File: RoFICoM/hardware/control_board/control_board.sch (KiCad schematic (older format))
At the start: 26 parts, among them J1 Skirt Cable, J2 M+, J3 M-, J4 SWD, J5 DBG_UART, J6 SYS_CON, J7 SLIDER, U1 STM32G071GBU6, U2 DRV8837C, U3 BU52272NUZ, U4 MIC5365, U5 BU52272NUZ

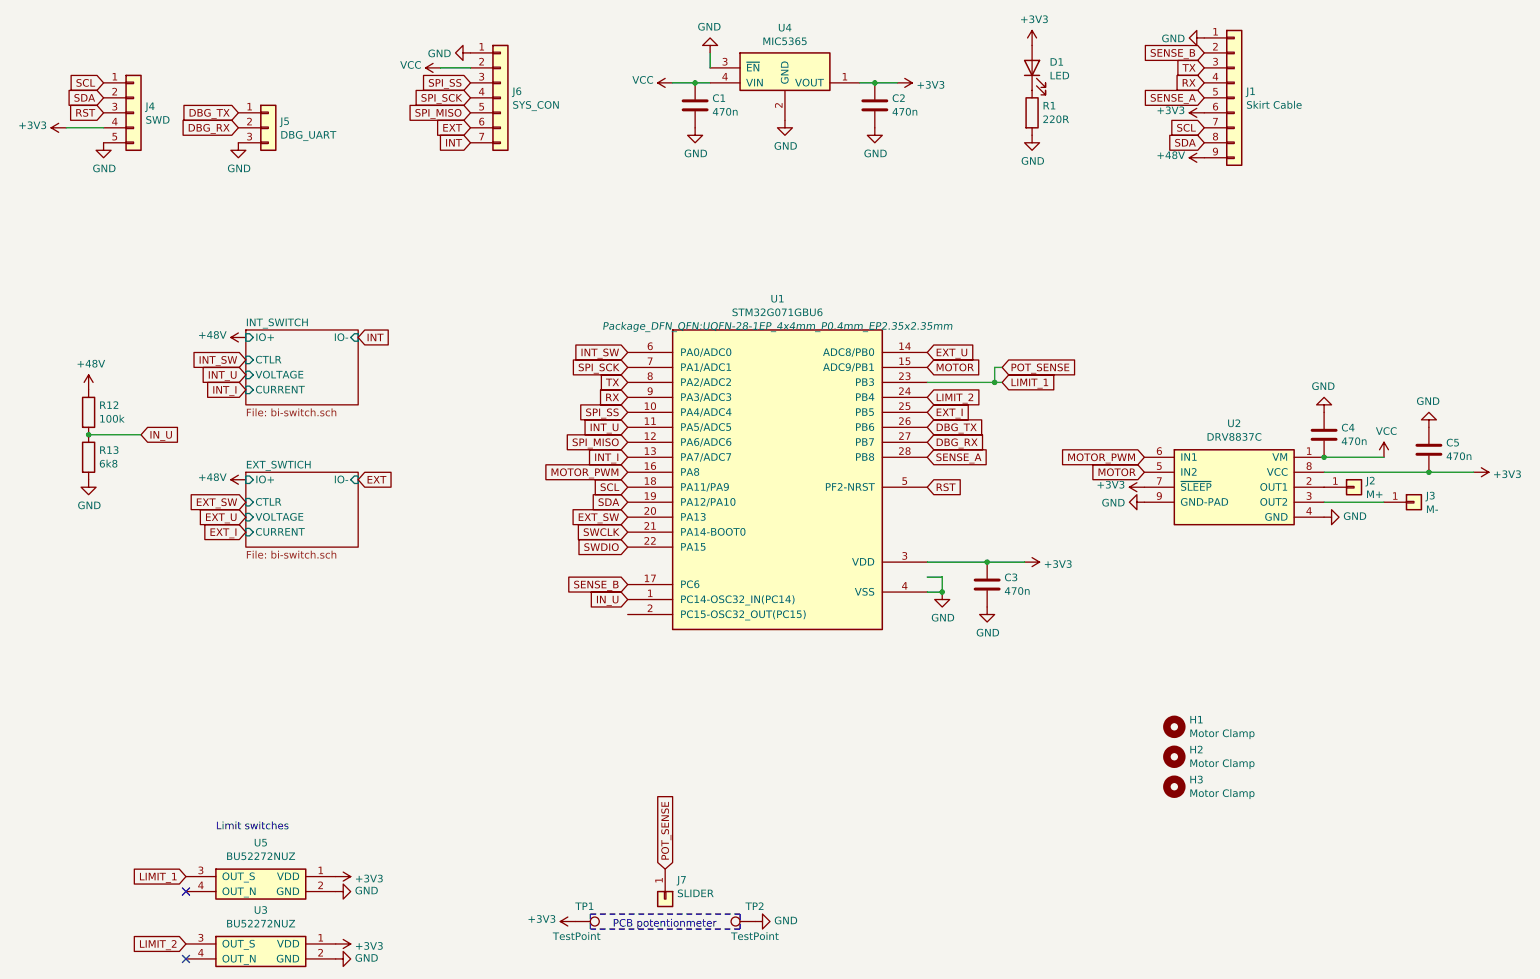
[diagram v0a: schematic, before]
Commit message: RoFICoM: Route ContorlBoard v0.2
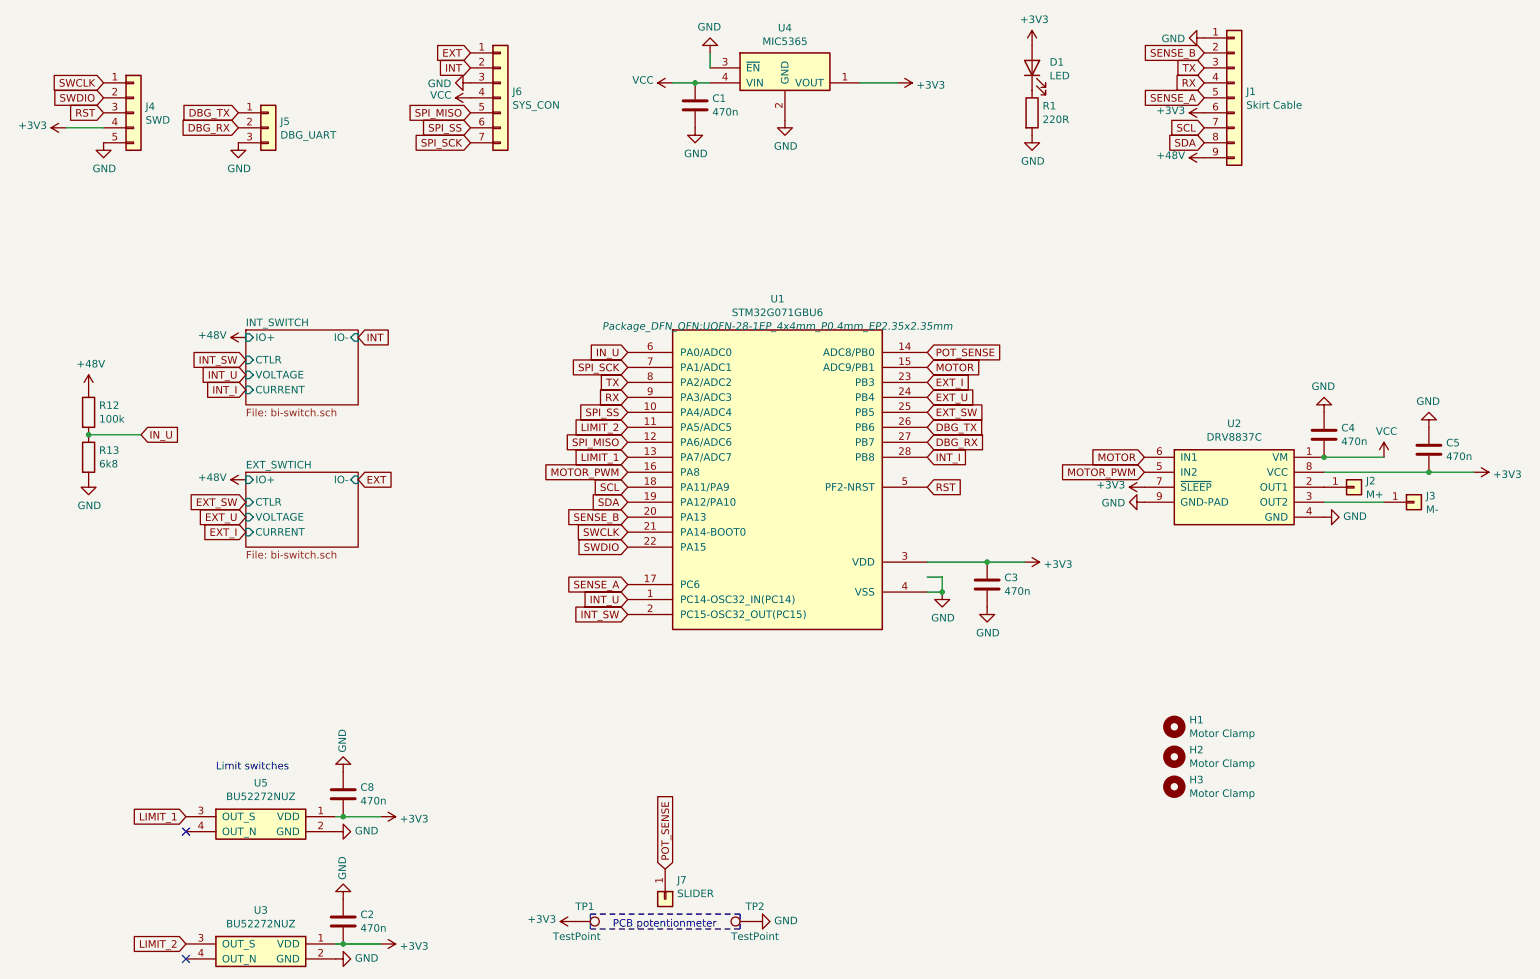
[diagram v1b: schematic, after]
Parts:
- added C8: 470n, Capacitor_SMD:C_0402_1005Metric, symbol Device:C
- J4: footprint Connector_PinHeader_1.27mm:PinHeader_1x05_P1.27mm_Vertical -> Connector_PinHeader_2.54mm:PinHeader_1x05_P2.54mm_Vertical
- J5: footprint Connector_PinHeader_1.27mm:PinHeader_1x03_P1.27mm_Vertical -> Connector_PinSocket_2.54mm:PinSocket_1x03_P2.54mm_Vertical
- J6: footprint Connector_PinHeader_1.27mm:PinHeader_1x07_P1.27mm_Vertical -> rofi:pogo_row_4_3
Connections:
- wire segments 21 -> 19
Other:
- moved on the sheet: C2, U5
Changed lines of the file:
@@
 L Device:C C2
 U 1 1 5C86BCA3
-P 6350 1550
-F 0 "C2" H 6465 1596 50  0000 L CNN
-F 1 "470n" H 6465 1505 50  0000 L CNN
-F 2 "Capacitor_SMD:C_0402_1005Metric" H 6388 1400 50  0001 C CNN
-F 3 "~" H 6350 1550 50  0001 C CNN
-	1    6350 1550
-	1    0    0    -1
-$EndComp
-Wire Wire Line
-	6500 1400 6350 1400
-Wire Wire Line
-	6350 1400 6250 1400
-Connection ~ 6350 1400
-$Comp
-L power:GND #PWR0108
-U 1 1 5C86BD54
-P 6350 1700
-F 0 "#PWR0108" H 6350 1450 50  0001 C CNN
-F 1 "GND" H 6355 1527 50  0000 C CNN
-F 2 "" H 6350 1700 50  0001 C CNN
-F 3 "" H 6350 1700 50  0001 C CNN
-	1    6350 1700
+P 2800 7000
+F 0 "C2" H 2915 7046 50  0000 L CNN
+F 1 "470n" H 2915 6955 50  0000 L CNN
+F 2 "Capacitor_SMD:C_0402_1005Metric" H 2838 6850 50  0001 C CNN
+F 3 "~" H 2800 7000 50  0001 C CNN
+	1    2800 7000
 	1    0    0    -1
 $EndComp
@@
 	0    1    1    0
 $EndComp
+Text GLabel 8150 3900 0    50   Input ~ 0
+MOTOR
 Text GLabel 8150 4000 0    50   Input ~ 0
-MOTOR
-Text GLabel 8150 3900 0    50   Input ~ 0
 MOTOR_PWM
 $Comp
@@
 L power:+3V3 #PWR0120
 U 1 1 5C86D9DD
-P 2750 7150
-F 0 "#PWR0120" H 2750 7000 50  0001 C CNN
-F 1 "+3V3" V 2765 7278 50  0000 L CNN
-F 2 "" H 2750 7150 50  0001 C CNN
-F 3 "" H 2750 7150 50  0001 C CNN
-	1    2750 7150
+P 3050 7150
+F 0 "#PWR0120" H 3050 7000 50  0001 C CNN
+F 1 "+3V3" V 3065 7278 50  0000 L CNN
+F 2 "" H 3050 7150 50  0001 C CNN
+F 3 "" H 3050 7150 50  0001 C CNN
+	1    3050 7150
 	0    1    1    0
 $EndComp
@@
 Text GLabel 1200 1600 0    50   Input ~ 0
 RST
-Text GLabel 1200 1500 0    50   Input ~ 0
-SDA
-Text GLabel 1200 1400 0    50   Input ~ 0
-SCL
 $Comp
 L Connector_Generic:Conn_01x05 J4
@@
 F 0 "J4" H 1480 1642 50  0000 L CNN
 F 1 "SWD" H 1480 1551 50  0000 L CNN
-F 2 "Connector_PinHeader_1.27mm:PinHeader_1x05_P1.27mm_Vertical" H 1400 1600 50  0001 C CNN
+F 2 "Connector_PinHeader_2.54mm:PinHeader_1x05_P2.54mm_Vertical" H 1400 1600 50  0001 C CNN
 F 3 "~" H 1400 1600 50  0001 C CNN
 	1    1400 1600
@@
 L rofi:BU52272NUZ U5
 U 1 1 5C86EF3E
-P 2250 6750
-F 0 "U5" H 2250 7025 50  0000 C CNN
-F 1 "BU52272NUZ" H 2250 6934 50  0000 C CNN
-F 2 "rofi:VSON04Z1114A" H 2250 6750 50  0001 C CNN
-F 3 "" H 2250 6750 50  0001 C CNN
-	1    2250 6750
+P 2250 6350
+F 0 "U5" H 2250 6625 50  0000 C CNN
+F 1 "BU52272NUZ" H 2250 6534 50  0000 C CNN
+F 2 "rofi:VSON04Z1114A" H 2250 6350 50  0001 C CNN
+F 3 "" H 2250 6350 50  0001 C CNN
+	1    2250 6350
 	1    0    0    -1
 $EndComp
@@
 L power:+3V3 #PWR0124
 U 1 1 5C86EF44
-P 2750 6700
-F 0 "#PWR0124" H 2750 6550 50  0001 C CNN
-F 1 "+3V3" V 2765 6828 50  0000 L CNN
-F 2 "" H 2750 6700 50  0001 C CNN
-F 3 "" H 2750 6700 50  0001 C CNN
-	1    2750 6700
+P 3050 6300
+F 0 "#PWR0124" H 3050 6150 50  0001 C CNN
+F 1 "+3V3" V 3065 6428 50  0000 L CNN
+F 2 "" H 3050 6300 50  0001 C CNN
+F 3 "" H 3050 6300 50  0001 C CNN
+	1    3050 6300
 	0    1    1    0
 $EndComp
@@
 L power:GND #PWR0125
 U 1 1 5C86EF4A
-P 2750 6800
-F 0 "#PWR0125" H 2750 6550 50  0001 C CNN
-F 1 "GND" V 2755 6672 50  0000 R CNN
-F 2 "" H 2750 6800 50  0001 C CNN
-F 3 "" H 2750 6800 50  0001 C CNN
-	1    2750 6800
-	0    -1   -1   0
-$EndComp
-Text GLabel 1750 6700 0    50   Input ~ 0
+P 2750 6400
+F 0 "#PWR0125" H 2750 6150 50  0001 C CNN
+F 1 "GND" V 2755 6272 50  0000 R CNN
+F 2 "" H 2750 6400 50  0001 C CNN
+F 3 "" H 2750 6400 50  0001 C CNN
+	1    2750 6400
+	0    -1   -1   0
+$EndComp
+Text GLabel 1750 6300 0    50   Input ~ 0
 LIMIT_1
 Text GLabel 1750 7150 0    50   Input ~ 0
 LIMIT_2
-NoConn ~ 1750 6800
+NoConn ~ 1750 6400
 NoConn ~ 1750 7250
-Text GLabel 7200 3400 2    50   Input ~ 0
+Text GLabel 4700 3900 0    50   Input ~ 0
 LIMIT_1
-Text GLabel 6700 3500 2    50   Input ~ 0
+Text GLabel 4700 3700 0    50   Input ~ 0
 LIMIT_2
-Wire Wire Line
-	7200 3400 7150 3400
-Wire Wire Line
-	7150 3300 7200 3300
-Wire Wire Line
-	7150 3300 7150 3400
-Connection ~ 7150 3400
-Wire Wire Line
-	7150 3400 6700 3400
-Text GLabel 7200 3300 2    50   Input ~ 0
+Text GLabel 6700 3200 2    50   Input ~ 0
 POT_SENSE
 $Comp
@@
 	1    0    0    -1
 $EndComp
+Text GLabel 4700 4950 0    50   Input ~ 0
+INT_SW
+Text GLabel 4700 4850 0    50   Input ~ 0
+INT_U
+Text GLabel 6700 3900 2    50   Input ~ 0
+INT_I
+Text GLabel 6700 3600 2    50   Input ~ 0
+EXT_SW
+Text GLabel 6700 3500 2    50   Input ~ 0
+EXT_U
+Text GLabel 6700 3400 2    50   Input ~ 0
+EXT_I
+Text GLabel 4700 4750 0    50   Input ~ 0
+SENSE_A
+Text GLabel 4700 4300 0    50   Input ~ 0
+SENSE_B
 Text GLabel 4700 3200 0    50   Input ~ 0
-INT_SW
-Text GLabel 4700 3700 0    50   Input ~ 0
-INT_U
-Text GLabel 4700 3900 0    50   Input ~ 0
-INT_I
-Text GLabel 4700 4300 0    50   Input ~ 0
-EXT_SW
-Text GLabel 6700 3200 2    50   Input ~ 0
-EXT_U
-Text GLabel 6700 3600 2    50   Input ~ 0
-EXT_I
-Text GLabel 6700 3900 2    50   Input ~ 0
-SENSE_A
-Text GLabel 4700 4750 0    50   Input ~ 0
-SENSE_B
-Text GLabel 4700 4850 0    50   Input ~ 0
 IN_U
 $Sheet
@@
 	0    -1   -1   0
 $EndComp
-Text Notes 1950 6400 0    50   ~ 0
+Text Notes 1950 6000 0    50   ~ 0
 Limit switches
 $Comp
@@
 F 0 "J5" H 2380 1742 50  0000 L CNN
 F 1 "DBG_UART" H 2380 1651 50  0000 L CNN
-F 2 "Connector_PinHeader_1.27mm:PinHeader_1x03_P1.27mm_Vertical" H 2300 1700 50  0001 C CNN
+F 2 "Connector_PinSocket_2.54mm:PinSocket_1x03_P2.54mm_Vertical" H 2300 1700 50  0001 C CNN
 F 3 "~" H 2300 1700 50  0001 C CNN
 	1    2300 1700
@@
 F 0 "J6" H 3930 1542 50  0000 L CNN
 F 1 "SYS_CON" H 3930 1451 50  0000 L CNN
-F 2 "Connector_PinHeader_1.27mm:PinHeader_1x07_P1.27mm_Vertical" H 3850 1500 50  0001 C CNN
+F 2 "rofi:pogo_row_4_3" H 3850 1500 50  0001 C CNN
 F 3 "~" H 3850 1500 50  0001 C CNN
 	1    3850 1500
 	1    0    0    -1
 $EndComp
-Text GLabel 3650 1800 0    50   Input ~ 0
+Text GLabel 3650 1300 0    50   Input ~ 0
 INT
-Text GLabel 3650 1700 0    50   Input ~ 0
+Text GLabel 3650 1200 0    50   Input ~ 0
 EXT
 $Comp
 L power:GND #PWR0145
 U 1 1 5C8876CF
-P 3650 1200
-F 0 "#PWR0145" H 3650 950 50  0001 C CNN
-F 1 "GND" V 3655 1072 50  0000 R CNN
-F 2 "" H 3650 1200 50  0001 C CNN
-F 3 "" H 3650 1200 50  0001 C CNN
-	1    3650 1200
+P 3650 1400
+F 0 "#PWR0145" H 3650 1150 50  0001 C CNN
+F 1 "GND" V 3655 1272 50  0000 R CNN
+F 2 "" H 3650 1400 50  0001 C CNN
+F 3 "" H 3650 1400 50  0001 C CNN
+	1    3650 1400
 	0    1    1    0
 $EndComp
@@
 L power:VCC #PWR0146
 U 1 1 5C887716
-P 3450 1300
-F 0 "#PWR0146" H 3450 1150 50  0001 C CNN
-F 1 "VCC" V 3468 1427 50  0000 L CNN
-F 2 "" H 3450 1300 50  0001 C CNN
-F 3 "" H 3450 1300 50  0001 C CNN
-	1    3450 1300
-	0    -1   -1   0
-$EndComp
-Wire Wire Line
-	3450 1300 3650 1300
-Text GLabel 3650 1400 0    50   Input ~ 0
+P 3650 1500
+F 0 "#PWR0146" H 3650 1350 50  0001 C CNN
+F 1 "VCC" V 3668 1627 50  0000 L CNN
+F 2 "" H 3650 1500 50  0001 C CNN
+F 3 "" H 3650 1500 50  0001 C CNN
+	1    3650 1500
+	0    -1   -1   0
+$EndComp
+Text GLabel 3650 1700 0    50   Input ~ 0
 SPI_SS
-Text GLabel 3650 1500 0    50   Input ~ 0
+Text GLabel 3650 1800 0    50   Input ~ 0
 SPI_SCK
 Text GLabel 3650 1600 0    50   Input ~ 0
@@
 	1    0    0    -1
 $EndComp
+Text GLabel 1200 1400 0    50   Input ~ 0
+SWCLK
+Text GLabel 1200 1500 0    50   Input ~ 0
+SWDIO
+Wire Wire Line
+	3050 6300 2800 6300
+Wire Wire Line
+	3050 7150 2800 7150
+$Comp
+L Device:C C8
+U 1 1 5C890AED
+P 2800 6150
+F 0 "C8" H 2915 6196 50  0000 L CNN
+F 1 "470n" H 2915 6105 50  0000 L CNN
+F 2 "Capacitor_SMD:C_0402_1005Metric" H 2838 6000 50  0001 C CNN
+F 3 "~" H 2800 6150 50  0001 C CNN
+	1    2800 6150
+	1    0    0    -1
+$EndComp
+Connection ~ 2800 6300
+Wire Wire Line
+	2800 6300 2750 6300
+$Comp
+L power:GND #PWR0108
+U 1 1 5C890C98
+P 2800 6000
+F 0 "#PWR0108" H 2800 5750 50  0001 C CNN
+F 1 "GND" V 2805 5872 50  0000 R CNN
+F 2 "" H 2800 6000 50  0001 C CNN
+F 3 "" H 2800 6000 50  0001 C CNN
+	1    2800 6000
+	-1   0    0    1
+$EndComp
+Connection ~ 2800 7150
+Wire Wire Line
+	2800 7150 2750 7150
+$Comp
+L power:GND #PWR0149
+U 1 1 5C890F51
+P 2800 6850
+F 0 "#PWR0149" H 2800 6600 50  0001 C CNN
+F 1 "GND" V 2805 6722 50  0000 R CNN
+F 2 "" H 2800 6850 50  0001 C CNN
+F 3 "" H 2800 6850 50  0001 C CNN
+	1    2800 6850
+	-1   0    0    1
+$EndComp
+Wire Wire Line
+	6250 1400 6500 1400
 $EndSCHEMATC
